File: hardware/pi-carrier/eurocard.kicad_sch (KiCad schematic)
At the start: 67 parts, among them J1 DIN41612_C96_male_ra_molliebus, J2 usb, J4 Conn_02x20_Odd_Even, J5 Conn_02x20_raspberry_pi4B, J7 button1, J8 button1, J9 Conn_02x05_Odd_Even, U1 SN74LVC1G07DBVR, U10 Lite-on LTP747KR, U11 TCAN332DR, U12 MCP2518FD, U2 TCAN332DR, U3 LM1117IMPX-3.3, U6 STM32F103C8T6, U8 SN74AHCT125PWR, U9 MAX7219CWG, X1 ASE-40.000MHz-LC, X2 ASE-8.000MHz-LC, Y1 ABS07-32.768KHZ-6-T

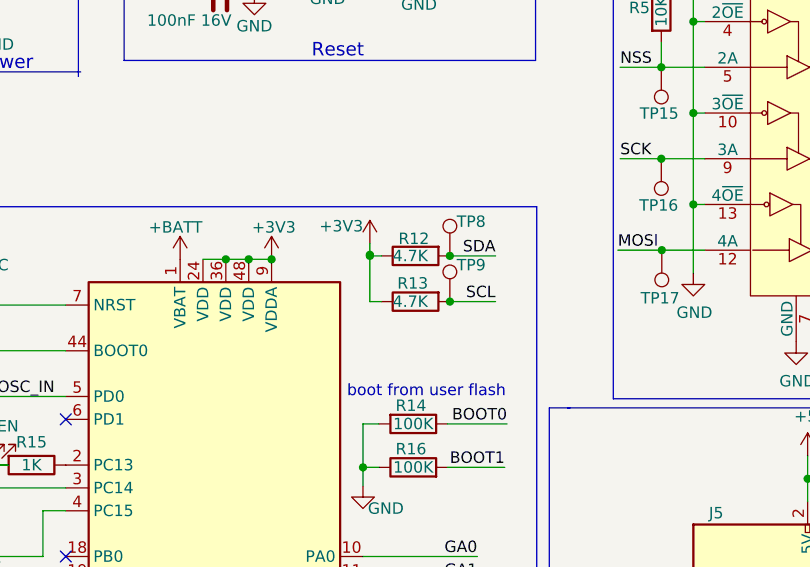
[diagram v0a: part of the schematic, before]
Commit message: pi-carrier: fix R12, R13 connection to +3V3
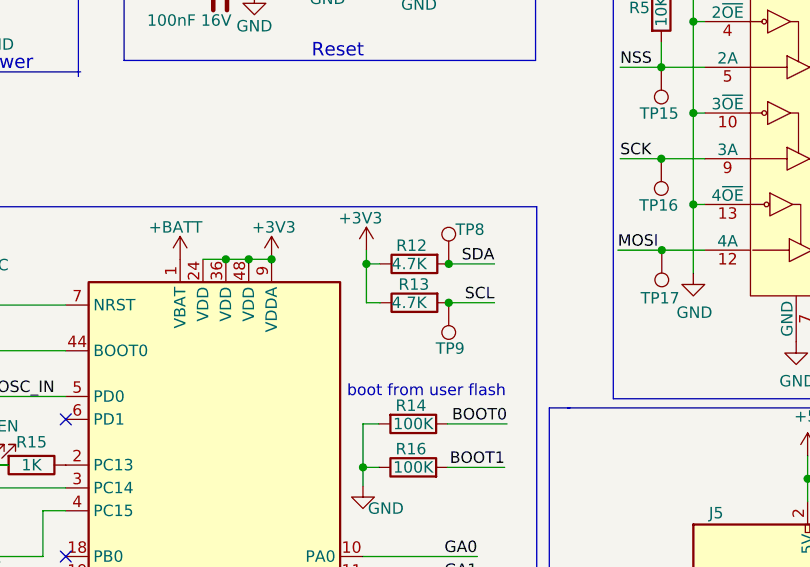
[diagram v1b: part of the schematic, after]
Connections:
- net +3V3: now also R12.1, R13.1
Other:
- moved on the sheet: R12, TP8, TP9
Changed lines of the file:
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@@
   (junction (at 65.405 135.89) (diameter 0) (color 0 0 0 0)
   )
-  (junction (at 148.209 69.215) (diameter 0) (color 0 0 0 0)
-  )
   (junction (at 261.62 27.94) (diameter 0) (color 0 0 0 0)
   )
@@
   (junction (at 125.857 69.596) (diameter 0) (color 0 0 0 0)
   )
+  (junction (at 148.082 70.104) (diameter 0) (color 0 0 0 0)
+  )
   (junction (at 98.552 30.48) (diameter 0) (color 0 0 0 0)
   )
   (junction (at 144.78 29.21) (diameter 0) (color 0 0 0 0)
   )
-  (junction (at 139.319 69.088) (diameter 0) (color 0 0 0 0)
-  )
   (junction (at 46.355 140.462) (diameter 0) (color 0 0 0 0)
   )
   (junction (at 71.247 193.294) (diameter 0) (color 0 0 0 0)
   )
-  (junction (at 139.319 69.215) (diameter 0) (color 0 0 0 0)
-  )
   (junction (at 187.96 165.1) (diameter 0) (color 0 0 0 0)
   )
@@
   (junction (at 81.28 21.59) (diameter 0) (color 0 0 0 0)
   )
+  (junction (at 138.938 70.104) (diameter 0) (color 0 0 0 0)
+  )
   (junction (at 83.947 76.708) (diameter 0) (color 0 0 0 0)
   )
@@
   (junction (at 237.49 154.94) (diameter 0) (color 0 0 0 0)
   )
-  (junction (at 148.209 74.295) (diameter 0) (color 0 0 0 0)
+  (junction (at 148.082 74.422) (diameter 0) (color 0 0 0 0)
   )
   (junction (at 95.25 30.48) (diameter 0) (color 0 0 0 0)
@@
     (stroke (width 0) (type default) (color 0 0 0 0))
   )
-  (wire (pts (xy 153.289 74.295) (xy 148.209 74.295))
+  (wire (pts (xy 153.162 74.422) (xy 148.082 74.422))
     (stroke (width 0) (type default) (color 0 0 0 0))
   )
@@
     (stroke (width 0) (type default) (color 0 0 0 0))
   )
+  (wire (pts (xy 138.938 74.422) (xy 140.462 74.422))
+    (stroke (width 0) (type default) (color 0 0 0 0))
+  )
   (wire (pts (xy 196.85 63.5) (xy 203.2 63.5))
     (stroke (width 0) (type default) (color 0 0 0 0))
@@
     (stroke (width 0) (type default) (color 0 0 0 0))
   )
-  (wire (pts (xy 139.319 69.215) (xy 139.319 74.295))
-    (stroke (width 0) (type default) (color 0 0 0 0))
-  )
   (polyline (pts (xy 65.532 14.986) (xy 41.402 14.986))
     (stroke (width 0) (type default) (color 0 0 0 0))
@@
     (stroke (width 0) (type default) (color 0 0 0 0))
   )
-  (wire (pts (xy 139.319 67.818) (xy 139.319 69.088))
-    (stroke (width 0) (type default) (color 0 0 0 0))
-  )
   (wire (pts (xy 123.317 145.796) (xy 123.317 147.066))
     (stroke (width 0) (type default) (color 0 0 0 0))
@@
     (stroke (width 0) (type default) (color 0 0 0 0))
   )
-  (wire (pts (xy 153.289 69.215) (xy 148.209 69.215))
+  (wire (pts (xy 153.162 70.104) (xy 148.082 70.104))
     (stroke (width 0) (type default) (color 0 0 0 0))
   )
@@
     (stroke (width 0) (type default) (color 0 0 0 0))
   )
-  (wire (pts (xy 139.319 74.295) (xy 140.589 74.295))
-    (stroke (width 0) (type default) (color 0 0 0 0))
-  )
   (polyline (pts (xy 57.404 156.718) (xy 157.226 156.718))
     (stroke (width 0) (type default) (color 0 0 0 0))
@@
     (stroke (width 0) (type default) (color 0 0 0 0))
   )
-  (wire (pts (xy 139.319 69.215) (xy 140.589 69.215))
-    (stroke (width 0) (type default) (color 0 0 0 0))
-  )
   (wire (pts (xy 251.46 127) (xy 266.7 127))
     (stroke (width 0) (type default) (color 0 0 0 0))
@@
     (stroke (width 0) (type default) (color 0 0 0 0))
   )
+  (wire (pts (xy 138.938 68.58) (xy 138.938 70.104))
+    (stroke (width 0) (type default) (color 0 0 0 0))
+  )
   (wire (pts (xy 251.46 144.78) (xy 266.7 144.78))
     (stroke (width 0) (type default) (color 0 0 0 0))
@@
     (stroke (width 0) (type default) (color 0 0 0 0))
   )
+  (wire (pts (xy 138.938 74.422) (xy 138.938 70.104))
+    (stroke (width 0) (type default) (color 0 0 0 0))
+  )
   (polyline (pts (xy 166.37 85.09) (xy 262.89 85.09))
     (stroke (width 0) (type default) (color 0 0 0 0))
@@
     (stroke (width 0) (type default) (color 0 0 0 0))
   )
+  (wire (pts (xy 138.938 70.104) (xy 140.462 70.104))
+    (stroke (width 0) (type default) (color 0 0 0 0))
+  )
   (wire (pts (xy 130.175 186.69) (xy 137.16 186.69))
     (stroke (width 0) (type default) (color 0 0 0 0))
@@
     (effects (font (size 1.27 1.27)) (justify left bottom))
   )
-  (label "SDA" (at 153.289 69.215 180)
+  (label "SDA" (at 153.162 70.104 180)
     (effects (font (size 1.27 1.27)) (justify right bottom))
   )
@@
     (effects (font (size 1.27 1.27)) (justify right bottom))
   )
-  (label "SCL" (at 153.289 74.295 180)
+  (label "SCL" (at 153.162 74.422 180)
     (effects (font (size 1.27 1.27)) (justify right bottom))
   )
@@
     (pin "1")
   )
-  (symbol (lib_id "Connector:TestPoint") (at 148.209 69.215 0) (unit 1)
+  (symbol (lib_id "Connector:TestPoint") (at 148.082 70.104 0) (unit 1)
     (in_bom yes) (on_board yes)
-    (property "Reference" "TP8" (id 0) (at 148.971 65.405 0)
+    (property "Reference" "TP8" (id 0) (at 148.844 66.294 0)
       (effects (font (size 1.27 1.27)) (justify left))
     )
-    (property "Value" "SDA" (id 1) (at 150.749 67.1829 0)
+    (property "Value" "SDA" (id 1) (at 150.622 68.0719 0)
       (effects (font (size 1.27 1.27)) (justify left) hide)
     )
-    (property "Footprint" "TestPoint:TestPoint_Pad_1.0x1.0mm" (id 2) (at 153.289 69.215 0)
+    (property "Footprint" "TestPoint:TestPoint_Pad_1.0x1.0mm" (id 2) (at 153.162 70.104 0)
       (effects (font (size 1.27 1.27)) hide)
     )
-    (property "Datasheet" "~" (id 3) (at 153.289 69.215 0)
+    (property "Datasheet" "~" (id 3) (at 153.162 70.104 0)
       (effects (font (size 1.27 1.27)) hide)
     )
@@
     (pin "1")
   )
-  (symbol (lib_id "Device:R") (at 144.399 69.215 90) (mirror x) (unit 1)
+  (symbol (lib_id "Device:R") (at 144.272 70.104 90) (mirror x) (unit 1)
     (in_bom yes) (on_board yes)
-    (property "Reference" "R12" (id 0) (at 142.494 67.31 90)
+    (property "Reference" "R12" (id 0) (at 142.24 68.072 90)
       (effects (font (size 1.27 1.27)) (justify right))
     )
-    (property "Value" "4.7K" (id 1) (at 141.859 69.215 90)
+    (property "Value" "4.7K" (id 1) (at 141.732 70.104 90)
       (effects (font (size 1.27 1.27)) (justify right))
     )
-    (property "Footprint" "Resistor_SMD:R_0603_1608Metric" (id 2) (at 144.399 67.437 90)
+    (property "Footprint" "Resistor_SMD:R_0603_1608Metric" (id 2) (at 144.272 68.326 90)
       (effects (font (size 1.27 1.27)) hide)
     )
-    (property "Datasheet" "~" (id 3) (at 144.399 69.215 0)
+    (property "Datasheet" "~" (id 3) (at 144.272 70.104 0)
       (effects (font (size 1.27 1.27)) hide)
     )
@@
     (pin "1")
   )
-  (symbol (lib_id "Device:R") (at 144.399 74.295 90) (mirror x) (unit 1)
+  (symbol (lib_id "Device:R") (at 144.272 74.422 90) (mirror x) (unit 1)
     (in_bom yes) (on_board yes)
-    (property "Reference" "R13" (id 0) (at 142.367 72.263 90)
+    (property "Reference" "R13" (id 0) (at 142.494 72.39 90)
       (effects (font (size 1.27 1.27)) (justify right))
     )
-    (property "Value" "4.7K" (id 1) (at 141.859 74.295 90)
+    (property "Value" "4.7K" (id 1) (at 141.732 74.422 90)
       (effects (font (size 1.27 1.27)) (justify right))
     )
-    (property "Footprint" "Resistor_SMD:R_0603_1608Metric" (id 2) (at 144.399 72.517 90)
+    (property "Footprint" "Resistor_SMD:R_0603_1608Metric" (id 2) (at 144.272 72.644 90)
       (effects (font (size 1.27 1.27)) hide)
     )
-    (property "Datasheet" "~" (id 3) (at 144.399 74.295 0)
+    (property "Datasheet" "~" (id 3) (at 144.272 74.422 0)
       (effects (font (size 1.27 1.27)) hide)
     )
@@
     (pin "2")
   )
-  (symbol (lib_id "Connector:TestPoint") (at 148.209 74.295 0) (unit 1)
+  (symbol (lib_id "Connector:TestPoint") (at 148.082 74.422 180) (unit 1)
     (in_bom yes) (on_board yes)
-    (property "Reference" "TP9" (id 0) (at 148.971 70.231 0)
+    (property "Reference" "TP9" (id 0) (at 149.86 79.502 0)
       (effects (font (size 1.27 1.27)) (justify left))
     )
-    (property "Value" "SCL" (id 1) (at 150.749 72.2629 0)
+    (property "Value" "SCL" (id 1) (at 145.542 76.4541 0)
       (effects (font (size 1.27 1.27)) (justify left) hide)
     )
-    (property "Footprint" "TestPoint:TestPoint_Pad_1.0x1.0mm" (id 2) (at 153.289 74.295 0)
+    (property "Footprint" "TestPoint:TestPoint_Pad_1.0x1.0mm" (id 2) (at 143.002 74.422 0)
       (effects (font (size 1.27 1.27)) hide)
     )
-    (property "Datasheet" "~" (id 3) (at 153.289 74.295 0)
+    (property "Datasheet" "~" (id 3) (at 143.002 74.422 0)
       (effects (font (size 1.27 1.27)) hide)
     )
@@
     (pin "1")
   )
-  (symbol (lib_id "power:+3V3") (at 139.319 67.818 0) (mirror y) (unit 1)
+  (symbol (lib_id "power:+3V3") (at 138.938 68.58 0) (mirror y) (unit 1)
     (in_bom yes) (on_board yes)
-    (property "Reference" "#PWR054" (id 0) (at 139.319 71.628 0)
+    (property "Reference" "#PWR054" (id 0) (at 138.938 72.39 0)
       (effects (font (size 1.27 1.27)) hide)
     )
-    (property "Value" "+3V3" (id 1) (at 136.144 65.913 0))
-    (property "Footprint" "" (id 2) (at 139.319 67.818 0)
+    (property "Value" "+3V3" (id 1) (at 138.2776 65.024 0))
+    (property "Footprint" "" (id 2) (at 138.938 68.58 0)
       (effects (font (size 1.27 1.27)) hide)
     )
-    (property "Datasheet" "" (id 3) (at 139.319 67.818 0)
+    (property "Datasheet" "" (id 3) (at 138.938 68.58 0)
       (effects (font (size 1.27 1.27)) hide)
     )

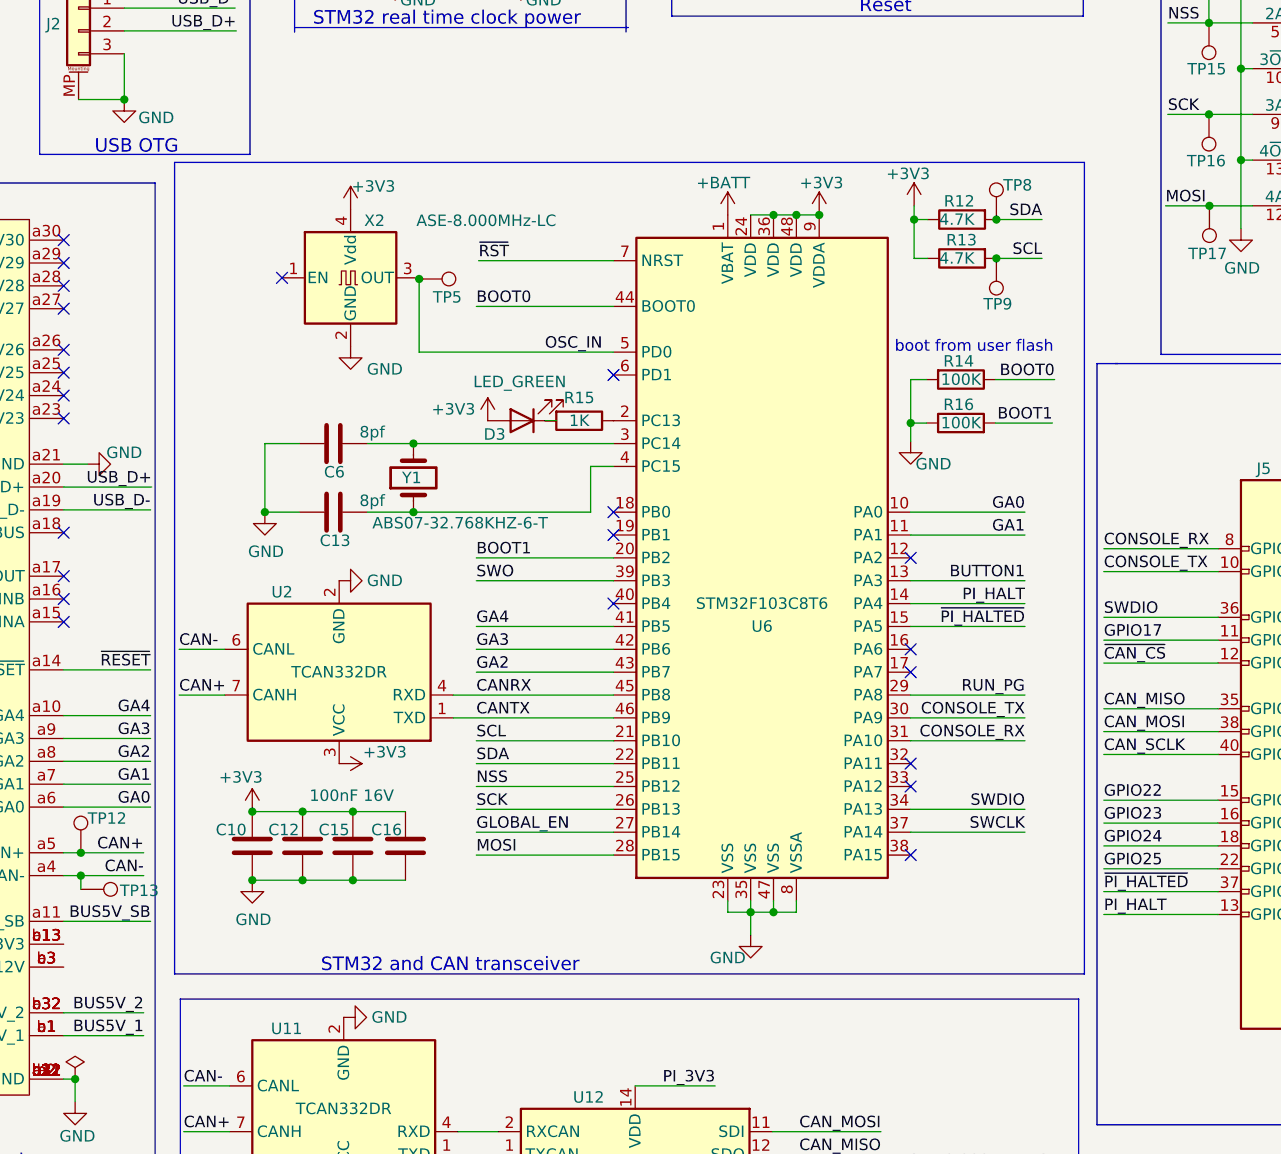
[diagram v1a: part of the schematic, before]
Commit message: pi-carrier: tweak test points
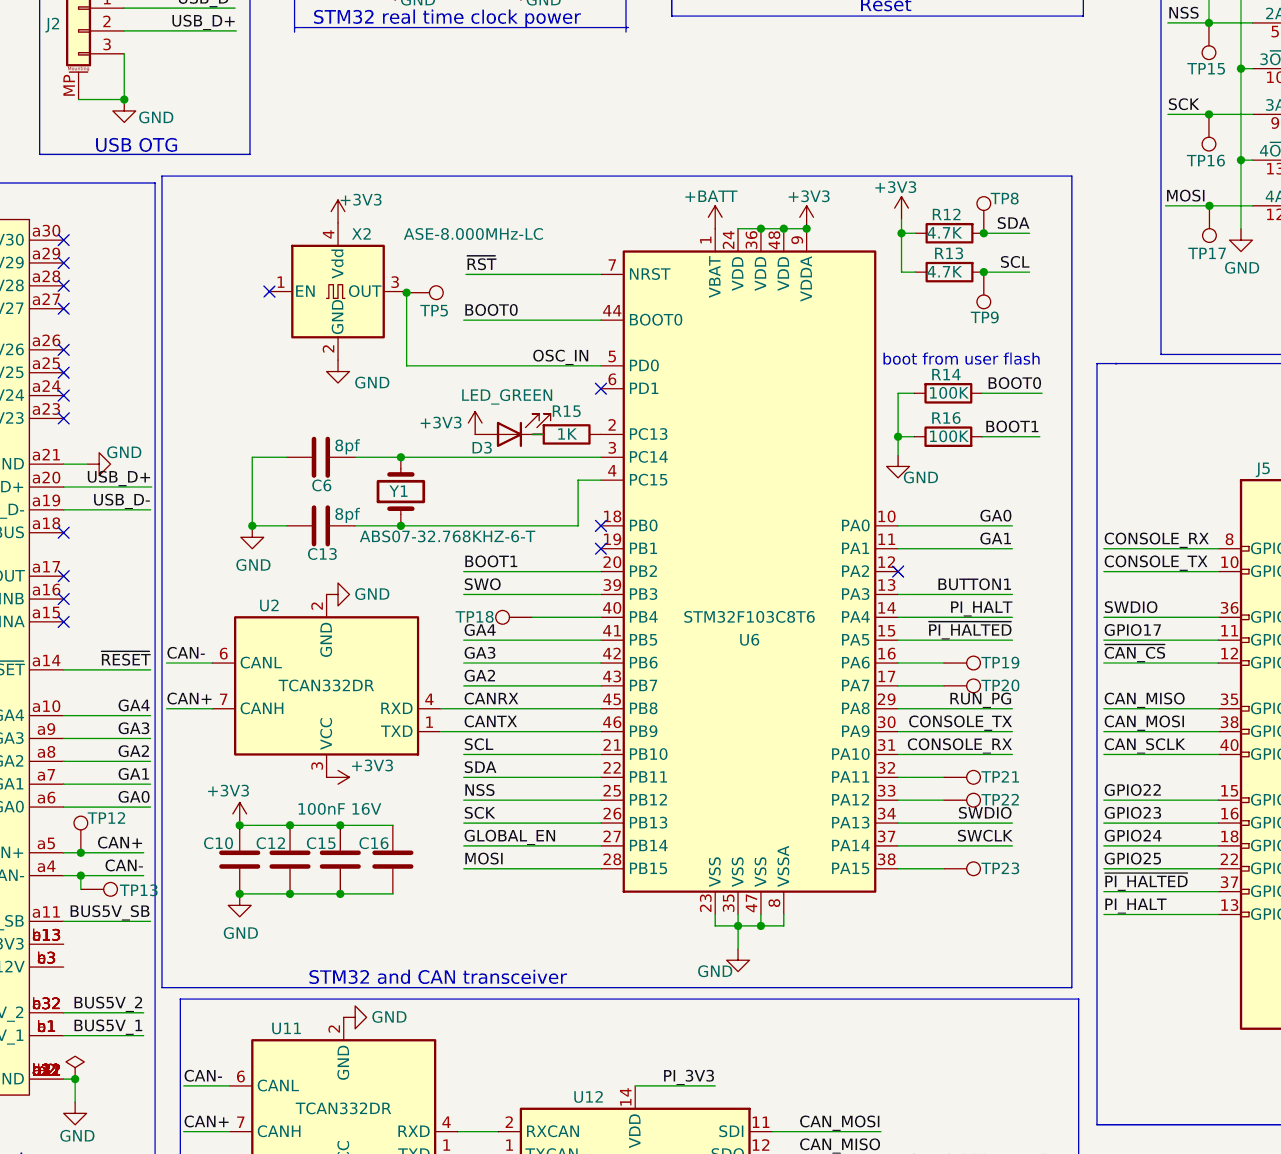
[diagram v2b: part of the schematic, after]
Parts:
- added TP18: PB4, TestPoint:TestPoint_Pad_1.0x1.0mm, symbol Connector:TestPoint
- added TP19: PA6, TestPoint:TestPoint_Pad_1.0x1.0mm, symbol Connector:TestPoint
- added TP20: PA7, TestPoint:TestPoint_Pad_1.0x1.0mm, symbol Connector:TestPoint
- added TP21: PA11, TestPoint:TestPoint_Pad_1.0x1.0mm, symbol Connector:TestPoint
- added TP22: PA12, TestPoint:TestPoint_Pad_1.0x1.0mm, symbol Connector:TestPoint
- added TP23: PA15, TestPoint:TestPoint_Pad_1.0x1.0mm, symbol Connector:TestPoint
- F1: footprint Fuse:Fuse_1812_4532Metric_Pad1.30x3.40mm_HandSolder -> Fuse:Fuse_1812_4532Metric
- TP3: value SB -> STBY
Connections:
- net at U6.16 (PA6): now also TP19.1
- net at U6.17 (PA7): now also TP20.1
- net at U6.32 (PA11): now also TP21.1
- net at U6.33 (PA12): now also TP22.1
- net at U6.38 (PA15): now also TP23.1
- net at U6.40 (PB4): now also TP18.1
- no-connect marks 58 -> 52
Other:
- moved on the sheet: C10, C12, C13, C15, C16, C6, D3, R12, R13, R14, R15, R16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
